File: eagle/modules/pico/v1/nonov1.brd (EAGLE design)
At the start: 93.3 x 53.3 mm, 41 parts, among them IC1 MEGA8-AI, IC3 ULN2803A, IC4 ULN2803A, J1 RJ12STRAIGHT-RS232-SERVER

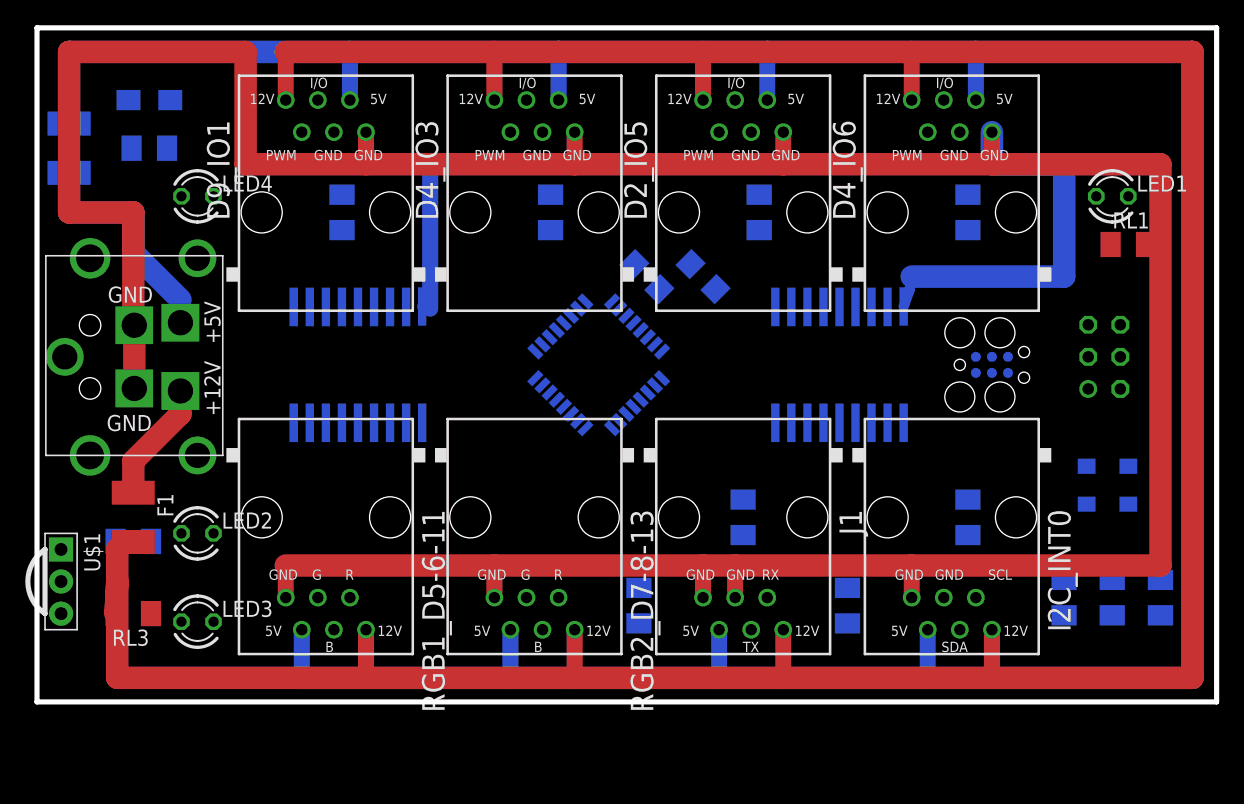
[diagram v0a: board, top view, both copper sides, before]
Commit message: Arduino ethernet first version
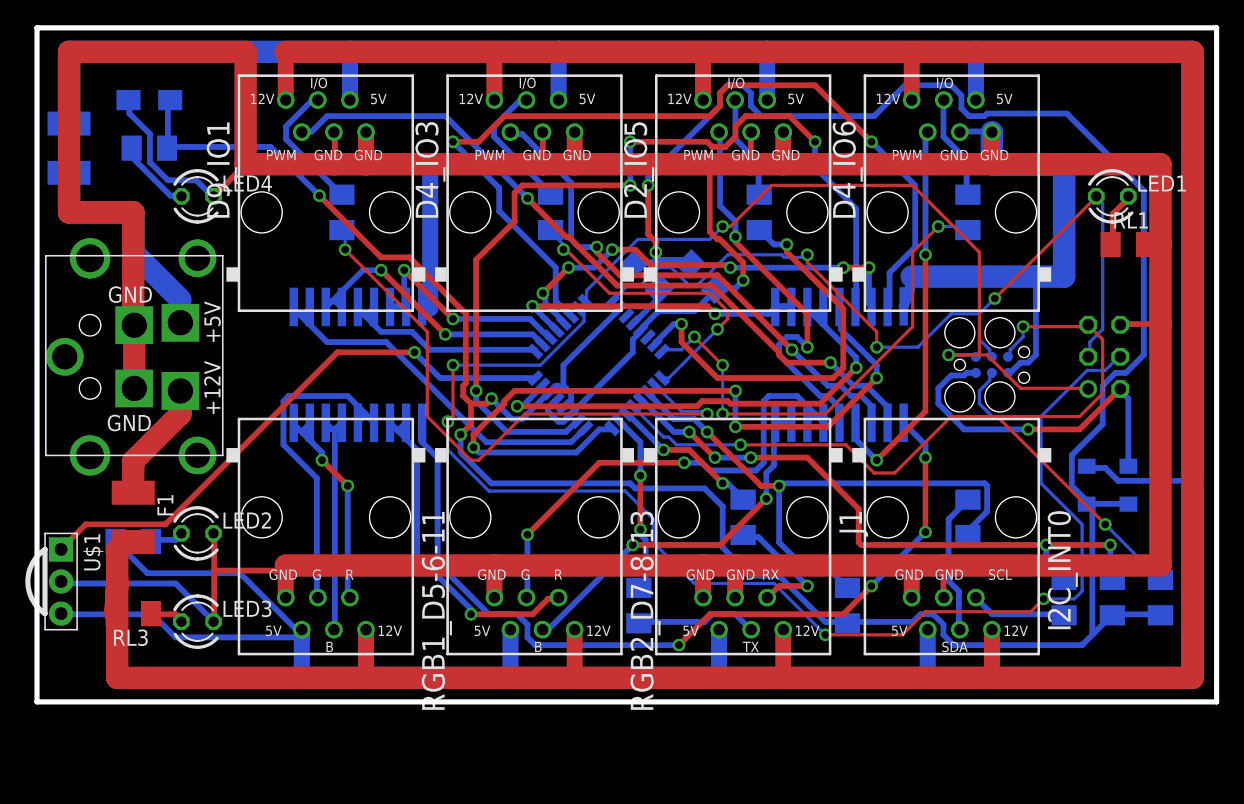
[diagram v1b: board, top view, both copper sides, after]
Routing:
- net 5V: track 0.00 -> 233.2 mm, vias 0 -> 5
- net MOSI: track 0.00 -> 110.3 mm, vias 0 -> 4
- net GND: track 301.8 -> 403.2 mm, vias 0 -> 1
- net RESET: track 0.00 -> 74.2 mm, vias 0 -> 3
- net D4: track 0.00 -> 71.6 mm, vias 0 -> 4
- net D10: track 0.00 -> 70.5 mm, vias 0 -> 2
- net SCK: track 0.00 -> 67.5 mm, vias 0 -> 3
- net COM: track 0.00 -> 66.6 mm, vias 0 -> 4
- net MISO: track 0.00 -> 60.2 mm, vias 0 -> 2
- net N$51: track 0.00 -> 57.8 mm, vias 0 -> 2
- net D2: track 0.00 -> 57.7 mm, vias 0 -> 4
- net SCL: track 0.00 -> 49.7 mm, vias 0 -> 5
- net A3: track 0.00 -> 47.7 mm, vias 0 -> 2
- net +5V: track 245.1 -> 291.4 mm
- net SDA: track 0.00 -> 46.2 mm, vias 0 -> 2
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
